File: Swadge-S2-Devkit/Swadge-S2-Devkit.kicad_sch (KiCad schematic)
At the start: 100 parts, among them J1 CurrentMonitor, J2 DEBUG_BANK_C, J3 DEBUG_BANK_B, J4 DEBUG_BANK_A, J5 MICSEL, J6 TRYMIC, J7 LEDK_J, J8 LCD18, J9 LCD28, M1 VZ43FC1B5640007L, P1 USB_C_Plug_USB2.0, Q1 Q_N_FET, Q2 AP2003_PN_FET, Q3 AP2003_PN_FET, Q4 AP2003_PN_FET, SW1 4-1437565-2, SW10 BLISTER_SILICONE_BUTTON, SW11 touch-ring-6, SW14 SW_SPDT, SW2 4-1437565-2, SW3 4-1437565-2, SW4 4-1437565-2, SW5 4-1437565-2, SW6 4-1437565-2, SW7 4-1437565-2, SW8 4-1437565-2, SW9 4-1437565-2, U1 ESP32-S2-SOLO, U10 GENERIC_LDO_2.8, U11 LCD_240x240_1.3_12, U12 LCD_135x240_1.14_13, U15 LCD_240x240_1.54_12, U2 BUS_PCIexpress, U3 MT3410, U4 GS321-TR, U5 QMA7981, U6 INGHAi_GSPK2308P-8R0.5W, U9 GENERIC_LDO_1.8

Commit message: Fixed warnings
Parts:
- C1, C10, C11, C12, C13, C14, C15, C16, C17, C18, C19, C2, C3, C4, C5, C6, C7, C8, C9, R1, R10, R11, R12, R13, R14, R15, R16, R17, R18, R19, R2, R20, R21, R22, R23, R24, R25, R26, R3, R4, R5, R6, R7, R8, R9: Notes 0603 Package -> (none)

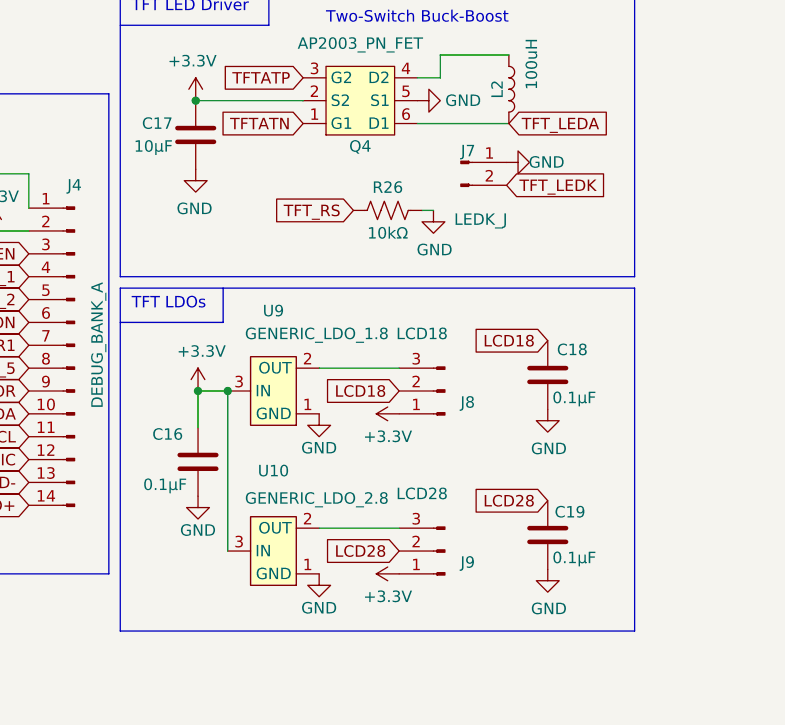
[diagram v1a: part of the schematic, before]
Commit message: Update note for manufacturing Add silkscreen version Ignore output folder
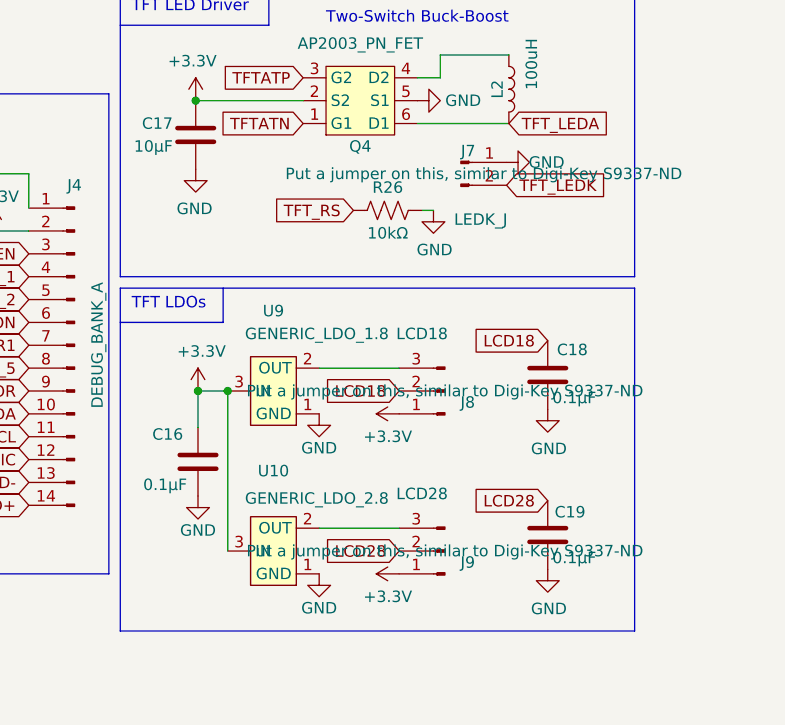
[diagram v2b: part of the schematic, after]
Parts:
- J7, J8, J9: Notes (none) -> Put a jumper on this, similar to Digi-Key S9337-ND
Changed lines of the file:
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@@
       (effects (font (size 1.27 1.27)) hide)
     )
-    (property "Notes" "" (id 7) (at 321.818 162.56 0))
+    (property "Notes" "Put a jumper on this, similar to Digi-Key S9337-ND" (id 7) (at 321.818 162.56 0))
     (pin "1")
     (pin "2")
@@
       (effects (font (size 1.27 1.27)) hide)
     )
-    (property "Notes" "" (id 7) (at 326.136 120.65 0))
+    (property "Notes" "Put a jumper on this, similar to Digi-Key S9337-ND" (id 7) (at 326.136 120.65 0))
     (pin "1")
     (pin "2")
@@
       (effects (font (size 1.27 1.27)) hide)
     )
-    (property "Notes" "" (id 7) (at 321.818 144.78 0))
-    (pin "1")
-    (pin "2")
+    (property "Notes" "Put a jumper on this, similar to Digi-Key S9337-ND" (id 7) (at 321.818 144.78 0))
+    (pin "1")
+    (pin "2")
